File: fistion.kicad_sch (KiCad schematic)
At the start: 37 parts, among them J1 debug-port, K1 diode-choc, K10 diode-choc, K11 diode-choc, K12 diode-choc, K13 diode-choc, K14 diode-choc, K15 diode-choc, K16 diode-choc, K2 diode-choc, K3 diode-choc, K4 diode-choc, K5 diode-choc, K6 diode-choc, K7 diode-choc, K8 diode-choc, K9 diode-choc, SW1 SW_Push, U1 MT25QL128ABA1ESE, U2 ms88sf3-nrf52840

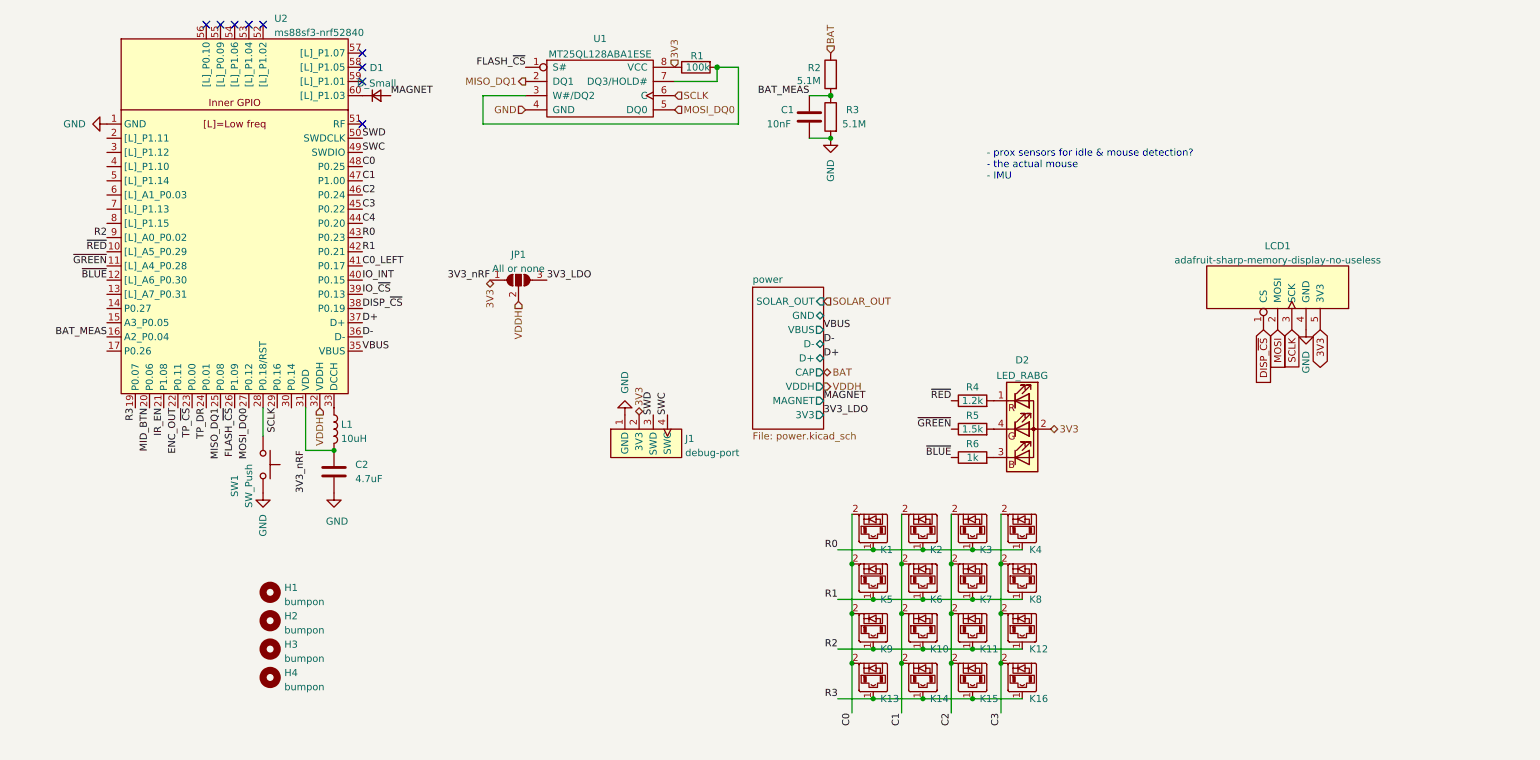
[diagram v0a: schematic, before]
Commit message: routed
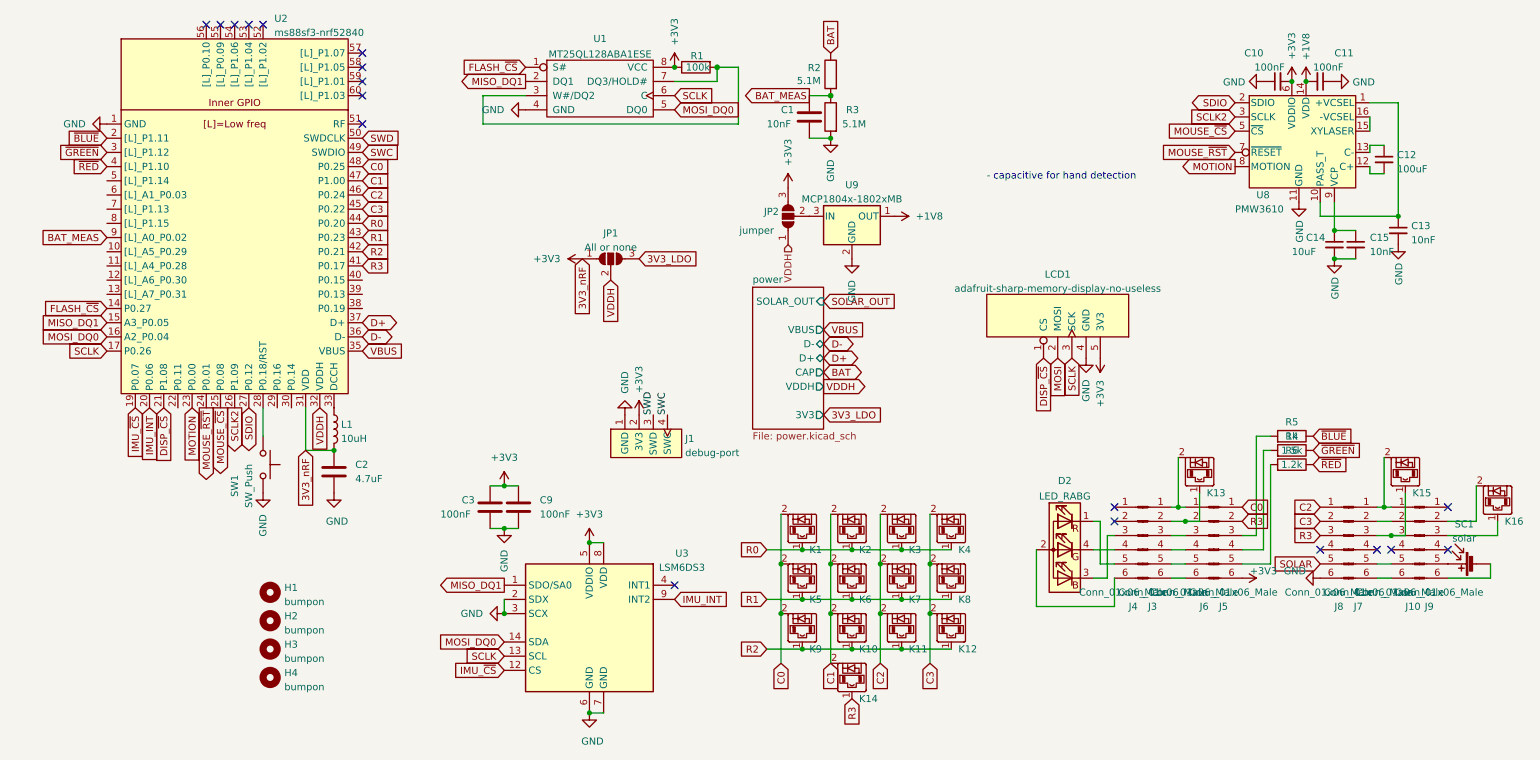
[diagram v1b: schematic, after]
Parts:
- removed D1: D_Small, Diode_SMD:D_SOD-123, symbol Device:D_Small
- added C10, C11: 100nF, Capacitor_SMD:C_0603_1608Metric, symbol Device:C_Small
- added C12: 100uF, Capacitor_SMD:C_0603_1608Metric, symbol Device:C_Small
- added C13, C15: 10nF, Capacitor_SMD:C_0603_1608Metric, symbol Device:C_Small
- added C14: 10uF, Capacitor_SMD:C_0603_1608Metric, symbol Device:C_Small
- added C3, C9: 100nF, Capacitor_SMD:C_0603_1608Metric, symbol Device:C
- added J10, J3, J4, J5, J6, J7, J8, J9: Conn_01x06_Male, fistion:bridge, symbol Connector:Conn_01x06_Male
- added JP2: jumper, Jumper:SolderJumper-3_P1.3mm_Open_RoundedPad1.0x1.5mm, symbol Jumper:SolderJumper_3_Open
- added SC1: solar, misc:KXOB25-05X3F, symbol Device:Solar_Cell
- added U3: LSM6DS3, Package_LGA:LGA-14_3x2.5mm_P0.5mm_LayoutBorder3x4y, symbol Sensor_Motion:LSM6DS3
- added U8: PMW3610, sensor:PMW3610, symbol sensor:PMW3610
- added U9: MCP1804x-1802xMB, Package_TO_SOT_SMD:SOT-89-3, symbol Regulator_Linear:MCP1804x-1802xMB
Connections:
- net C0_LEFT is gone; now on net R3: U2.41 (P0.17)
- net C4 is gone; now on net R0: U2.44 (P0.20)
- net IR_EN is gone; now on net DISP_~{CS}: U2.21 (P1.08)
- net BAT_MEAS: now also U2.9 ([L]_A0_P0.02); no longer U2.16 (A2_P0.04)
- net C0: now also J5.1 (Pin_1); no longer K13.2
- net C2: now also J8.1 (Pin_1); no longer K15.2
- net C3: now also J8.2 (Pin_2); no longer K16.2
- net DISP_~{CS}: no longer U2.38 (P0.19)
- net FLASH_~{CS}: now also U2.14 (P0.27); no longer U2.26 (P1.09)
- net GND: now also C10.1, C11.1, C13.2, C14.2, C15.2, C3.2, C9.2, J8.6 (Pin_6), U3.2 (SDX), U3.3 (SCX), U3.6 (GND), U3.7 (GND), U8.11 (GND), U9.2 (GND)
- net MISO_DQ1: now also U2.15 (A3_P0.05), U3.1 (SDO/SA0); no longer U2.25 (P0.08)
- net MOSI_DQ0: now also U2.16 (A2_P0.04), U3.14 (SDA); no longer U2.27 (P0.12)
- net R0: no longer U2.43 (P0.23)
- net R1: now also U2.43 (P0.23); no longer U2.42 (P0.21)
- net R2: now also U2.42 (P0.21); no longer U2.9 ([L]_A0_P0.02)
- net R3: now also J5.2 (Pin_2), J8.3 (Pin_3); no longer K13.1, K15.1, K16.1, U2.19 (P0.07)
- net SCLK: now also U2.17 (P0.26), U3.13 (SCL); no longer U2.29 (P0.16)
- net VDDH: now also JP2.1 (A)
- net ~{BLUE}: now also U2.2 ([L]_P1.11); no longer U2.12 ([L]_A6_P0.30)
- net ~{GREEN}: now also U2.3 ([L]_P1.12); no longer U2.11 ([L]_A4_P0.28)
- net ~{RED}: now also U2.4 ([L]_P1.10); no longer U2.10 ([L]_A5_P0.29)
- net at R4.2: now also J5.5 (Pin_5); no longer D2.1 (RK)
- net at R6.2: now also J5.3 (Pin_3); no longer D2.3 (BK)
- net at R5.2: now also J5.4 (Pin_4); no longer D2.4 (GK)
- net 3V3 renamed +3V3
- net +3V3: now also C10.2, C3.1, C9.1, J5.6 (Pin_6), JP2.3 (B), U3.5 (VDDIO), U3.8 (VDD), U8.6 (VDDIO); no longer D2.2 (A)
- net ENC_OUT: no longer names the net of U2.22 (P0.11)
- net IO_INT: no longer names the net of U2.40 (P0.15)
- net IO_~{CS}: no longer names the net of U2.39 (P0.13)
- net MID_BTN renamed IMU_INT
- net IMU_INT: now also U3.9 (INT2)
- net TP_DR renamed MOUSE_~{RST}
- net MOUSE_~{RST}: now also U8.7 (~{RESET})
- net TP_~{CS} renamed MOTION
- net MOTION: now also U8.8 (MOTION)
- new net: J9.3 (Pin_3), K16.1
- new net: J9.2 (Pin_2), K16.2
- new net: J3.1 (Pin_1), J6.1 (Pin_1), K13.2
- new net: J3.2 (Pin_2), J6.2 (Pin_2), K13.1
- new net: J3.3 (Pin_3), J6.3 (Pin_3)
- new net: J3.4 (Pin_4), J6.4 (Pin_4)
- new net: J3.5 (Pin_5), J6.5 (Pin_5)
- new net: J3.6 (Pin_6), J6.6 (Pin_6)
- new net: D2.3 (BK), J4.3 (Pin_3)
- new net: D2.4 (GK), J4.4 (Pin_4)
- new net: D2.1 (RK), J4.5 (Pin_5)
- new net: D2.2 (A), J4.6 (Pin_6)
- new net: J9.5 (Pin_5), SC1.1 (+)
- new net: J9.6 (Pin_6), SC1.2 (-)
- new net: C13.1, U8.1 (+VCSEL), U8.10 (PASS_T)
- new net: C12.2, U8.12 (C+)
- new net: C12.1, U8.13 (C-)
- new net: U8.15 (XYLASER), U8.16 (-VCSEL)
- new net: C14.1, C15.1, U8.9 (VCP)
- new net: J10.3 (Pin_3), J7.3 (Pin_3), K15.1
- new net: J10.1 (Pin_1), J7.1 (Pin_1), K15.2
- new net: JP2.2 (C), U9.3 (IN)
- new net: J10.2 (Pin_2), J7.2 (Pin_2)
- new net: J10.5 (Pin_5), J7.5 (Pin_5)
- new net: J10.6 (Pin_6), J7.6 (Pin_6)
- new net +1V8: C11.2, U8.14 (VDD), U9.1 (OUT)
- new net IMU_~{CS}: U2.19 (P0.07), U3.12 (CS)
- new net MOUSE_~{CS}: U2.25 (P0.08), U8.5 (~{CS})
- new net SCLK2: U2.26 (P1.09), U8.3 (SCLK)
- new net SDIO: U2.27 (P0.12), U8.2 (SDIO)
- new net SOLAR: J8.5 (Pin_5)
- no-connect marks 9 -> 18
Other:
- sheet power ports: added none; removed GND, MAGNET
- note added: "- capacitive for hand detection"
- note removed: "- prox sensors for idle & mouse detection? - the actual mouse - IMU"
- moved on the sheet: D2, JP1, K1, K10, K11, K12, K13, K14, K15, K16, K2, K3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
